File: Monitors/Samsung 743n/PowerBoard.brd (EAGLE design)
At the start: 160 x 128 mm, 60 parts, among them IC2 HV9961NG-G, T1 TRANS-1/1EFD25-10, X1 CON-MONPANEL, X2 CON-2MM-12P

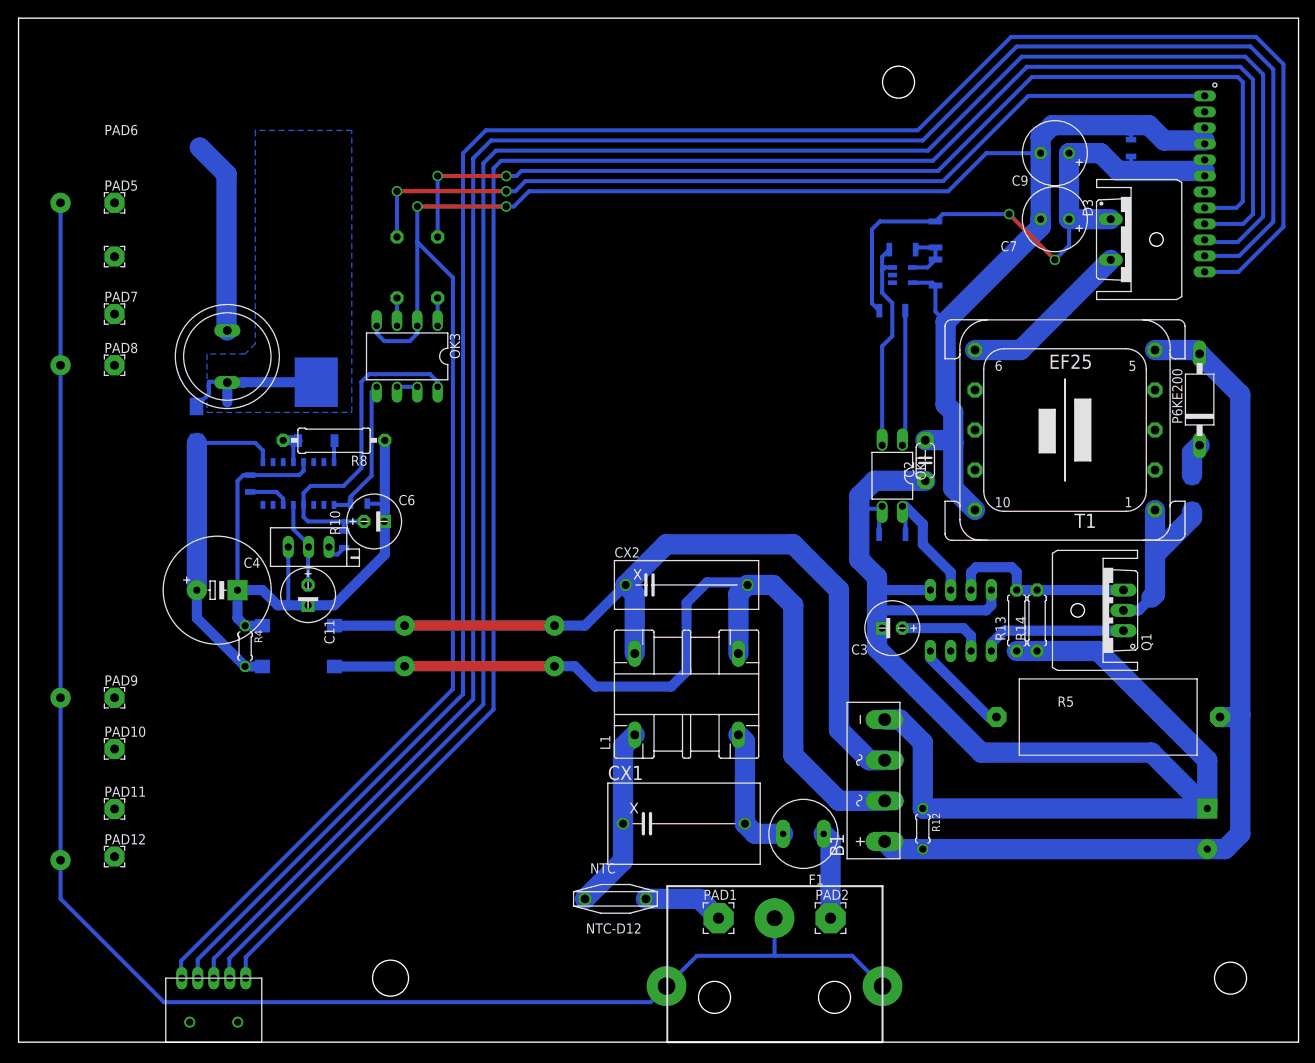
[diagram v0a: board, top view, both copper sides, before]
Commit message: Релиз
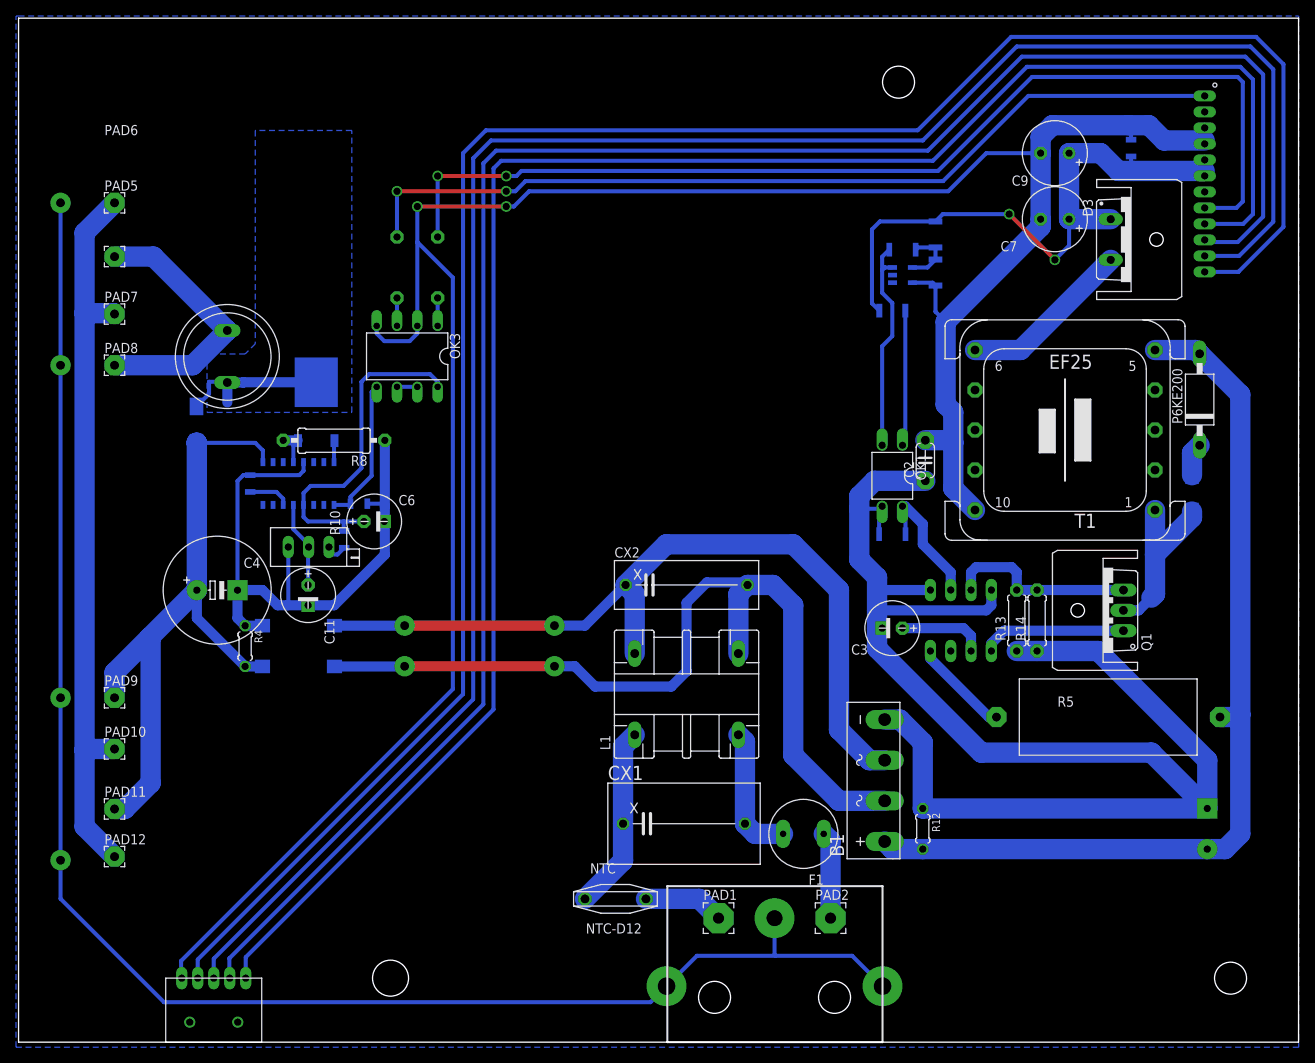
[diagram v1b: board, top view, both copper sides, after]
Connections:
- new net N$3: PAD10.1, PAD12.1, PAD5.1, PAD7.1
- net LED+: now also PAD11.1, PAD9.1
- net LED-: now also PAD6.1, PAD8.1
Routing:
- net N$3: track 0.00 -> 92.4 mm
- net LED+: track 42.7 -> 84.6 mm
- net LED-: track 24.3 -> 34.0 mm
- added copper zone on layer 16, net GROUND
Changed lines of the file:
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@@
 <wire x1="28.3225" y1="46.97" x2="22.29" y2="53.0025" width="1.27" layer="16"/>
 <wire x1="22.29" y1="53.0025" x2="22.29" y2="56.495" width="1.27" layer="16"/>
-<wire x1="22.29" y1="74.91" x2="22.245" y2="74.9325" width="0" layer="19" extent="16-16"/>
+<contactref element="PAD9" pad="1"/>
+<contactref element="PAD11" pad="1"/>
+<wire x1="12" y1="43.0475" x2="12" y2="46.205" width="2.54" layer="16"/>
+<wire x1="12" y1="46.205" x2="16.39375" y2="50.59875" width="2.54" layer="16"/>
+<wire x1="16.39375" y1="50.59875" x2="22.29" y2="56.495" width="2.54" layer="16"/>
+<wire x1="12" y1="29.1475" x2="13.2725" y2="29.1475" width="2.54" layer="16"/>
+<wire x1="13.2725" y1="29.1475" x2="16.51" y2="32.385" width="2.54" layer="16"/>
+<wire x1="16.51" y1="32.385" x2="16.51" y2="50.4825" width="2.54" layer="16"/>
+<wire x1="16.51" y1="50.4825" x2="16.39375" y2="50.59875" width="2.54" layer="16"/>
+<wire x1="22.245" y1="74.9325" x2="22.2675" y2="74.9325" width="2.54" layer="16"/>
+<wire x1="22.2675" y1="74.9325" x2="22.29" y2="74.91" width="2.54" layer="16"/>
 </signal>
 <signal name="LED-">
 <contactref element="L2" pad="P$2"/>
-<wire x1="22.65" y1="111.85" x2="26" y2="108.5" width="2.54" layer="16"/>
-<wire x1="26" y1="108.5" x2="26" y2="89.055" width="2.54" layer="16"/>
 <wire x1="26" y1="89.055" x2="26.1" y2="88.955" width="2.54" layer="16"/>
+<contactref element="PAD8" pad="1"/>
+<contactref element="PAD6" pad="1"/>
+<wire x1="26.1" y1="88.955" x2="16.8575" y2="98.1975" width="2.54" layer="16"/>
+<wire x1="16.8575" y1="98.1975" x2="12" y2="98.1975" width="2.54" layer="16"/>
+<wire x1="12" y1="84.615" x2="21.76" y2="84.615" width="2.54" layer="16"/>
+<wire x1="21.76" y1="84.615" x2="26.1" y2="88.955" width="2.54" layer="16"/>
 </signal>
 <signal name="N$7">
@@
 <wire x1="5.25" y1="17.9275" x2="18.1815" y2="4.996" width="0.508" layer="16"/>
 <wire x1="78.996" y1="4.996" x2="81" y2="7" width="0.508" layer="16"/>
+<polygon width="0.4064" layer="16" isolate="1.27" orphans="yes" rank="6">
+<vertex x="0" y="128.27"/>
+<vertex x="160.02" y="128.27"/>
+<vertex x="160.02" y="-0.635"/>
+<vertex x="-0.3175" y="-0.635"/>
+<vertex x="-0.3175" y="127.9525"/>
+<vertex x="-0.3175" y="128.27"/>
+</polygon>
 </signal>
 <signal name="K2">
@@
 <contactref element="X2" pad="7"/>
 </signal>
+<signal name="N$3">
+<contactref element="PAD7" pad="1"/>
+<contactref element="PAD5" pad="1"/>
+<contactref element="PAD10" pad="1"/>
+<contactref element="PAD12" pad="1"/>
+<wire x1="12" y1="104.915" x2="8.255" y2="101.17" width="2.54" layer="16"/>
+<wire x1="8.255" y1="26.9425" x2="12" y2="23.1975" width="2.54" layer="16"/>
+<wire x1="8.255" y1="101.17" x2="8.255" y2="91.1225" width="2.54" layer="16"/>
+<wire x1="8.255" y1="91.1225" x2="8.255" y2="36.5125" width="2.54" layer="16"/>
+<wire x1="8.255" y1="36.5125" x2="8.255" y2="26.9425" width="2.54" layer="16"/>
+<wire x1="12" y1="36.6475" x2="8.39" y2="36.6475" width="2.54" layer="16"/>
+<wire x1="8.39" y1="36.6475" x2="8.255" y2="36.5125" width="2.54" layer="16"/>
+<wire x1="12" y1="91.015" x2="11.8925" y2="91.1225" width="2.54" layer="16"/>
+<wire x1="11.8925" y1="91.1225" x2="8.255" y2="91.1225" width="2.54" layer="16"/>
+</signal>
 </signals>

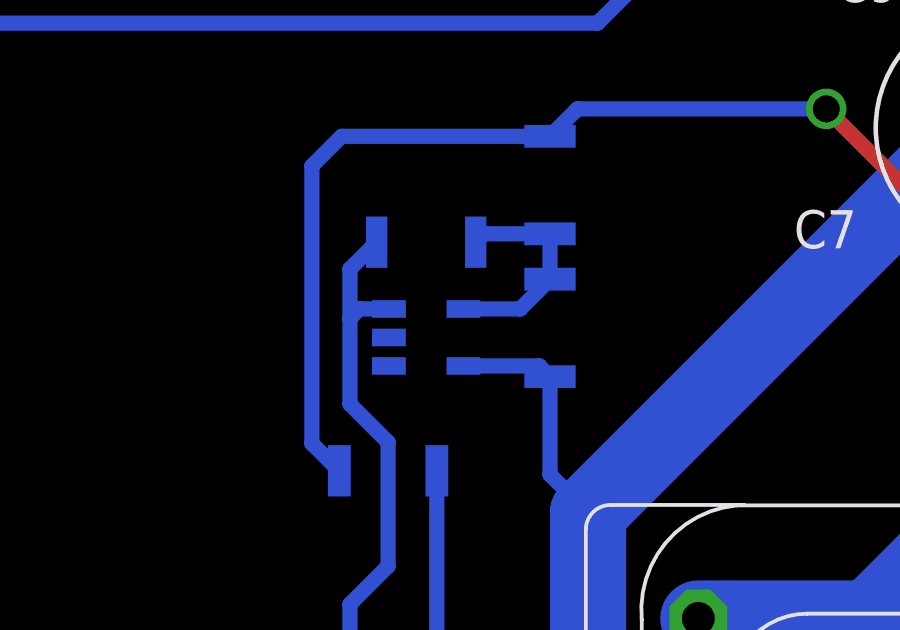
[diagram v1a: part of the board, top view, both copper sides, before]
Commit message: _)
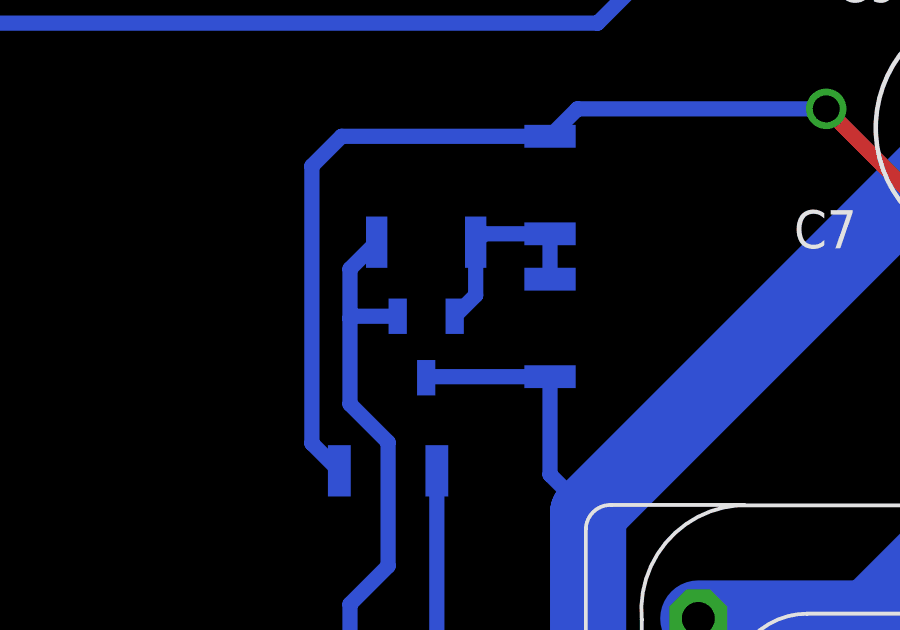
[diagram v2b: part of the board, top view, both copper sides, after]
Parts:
- U$3: value IC-TL431DBV -> IC-TL431CDBZR; device Flamberm:SOT95P280X145-5 -> Flamberm:SOT95P240X115-3
- moved U$3 0.32 mm to (110.5, 95.6), turned to 270 degrees
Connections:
- net GND: now also U$3.3; no longer U$3.5
- net N$23: now also U$3.2; no longer U$3.4
- net N$31: now also U$3.1; no longer U$3.3
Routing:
- net GND: track 302.6 -> 303.7 mm
- net N$23: track 7.40 -> 6.86 mm
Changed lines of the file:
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@@
 </layers>
 <board>
+<fusionsync huburn="a.cGVyc29uYWw6dWUyOGRlMGUz" projecturn="a.cGVyc29uYWw6dWUyOGRlMGUzIzIwMTgxMjA3MTY0MzUzMzMx" f3durn="urn:adsk.wipprod:dm.lineage:CbOk_p9-Sm28mP2tJHSDlw" pcbguid="25285c78-3eb6-47c6-8325-666efd53a6fb" lastpulledtime="" lastsyncedchangeguid="d28009d4-24da-5f07-1719-9be39d882890"/>
 <plain>
 <wire x1="0" y1="0" x2="160" y2="0" width="0" layer="20"/>
@@
 <attribute name="VALUE" x="132.6642" y="106.0958" size="1.27" layer="27" ratio="10" rot="R180"/>
 </element>
-<element name="U$3" library="Flamberm" library_urn="urn:adsk.eagle:library:2654185" package="SOT95P280X145-5" package3d_urn="urn:adsk.eagle:package:4135333/1" value="IC-TL431DBV" x="110.49" y="95.885" smashed="yes" rot="MR180">
-<attribute name="NAME" x="108.712" y="98.933" size="1.27" layer="26" ratio="10" rot="MR270"/>
-<attribute name="VALUE" x="113.538" y="98.933" size="1.27" layer="28" ratio="10" rot="MR270"/>
+<element name="U$3" library="Flamberm" library_urn="urn:adsk.eagle:library:2654185" package="SOT95P240X115-3" package3d_urn="urn:adsk.eagle:package:4135509/1" value="IC-TL431CDBZR" x="110.49" y="95.5675" smashed="yes" rot="MR270">
+<attribute name="NAME" x="113.538" y="97.3455" size="1.27" layer="26" ratio="10" rot="MR0"/>
+<attribute name="VALUE" x="113.538" y="92.5195" size="1.27" layer="28" ratio="10" rot="MR0"/>
 </element>
 <element name="R7" library="Flamberm" library_urn="urn:adsk.eagle:library:2654185" package="RESC3216X60" package3d_urn="urn:adsk.eagle:package:4015759/1" value="220R" x="109.22" y="91.44" smashed="yes" rot="MR0">
@@
 <wire x1="49.8475" y1="88.5825" x2="49.8475" y2="89.535" width="0.508" layer="16"/>
 <contactref element="C2" pad="2"/>
-<contactref element="U$3" pad="5"/>
+<contactref element="U$3" pad="3"/>
 <contactref element="R18" pad="1"/>
 <contactref element="C7" pad="-"/>
@@
 <wire x1="114.6175" y1="94.5775" x2="114.6175" y2="91.313" width="0.508" layer="16"/>
 <wire x1="114.6175" y1="91.313" x2="115.8875" y2="90.043" width="0.508" layer="16"/>
-<wire x1="111.7321" y1="94.935" x2="114.26" y2="94.935" width="0.508" layer="16"/>
-<wire x1="114.26" y1="94.935" x2="114.6175" y2="94.5775" width="0.508" layer="16"/>
 <wire x1="127.762" y1="111.125" x2="120.9675" y2="111.125" width="0.508" layer="16"/>
 <wire x1="120.9675" y1="111.125" x2="116.205" y2="106.3625" width="0.508" layer="16"/>
@@
 <wire x1="63.8175" y1="106.3625" x2="61.9125" y2="104.4575" width="0.508" layer="16"/>
 <wire x1="60.96" y1="104.4575" x2="49.8475" y2="104.4575" width="0.508" layer="1"/>
+<wire x1="114.6175" y1="94.5775" x2="110.5245" y2="94.5775" width="0.508" layer="16"/>
+<wire x1="110.5245" y1="94.5775" x2="110.49" y2="94.543" width="0.508" layer="16"/>
 </signal>
 <signal name="+5V">
@@
 <signal name="N$31">
 <contactref element="OK1" pad="2"/>
-<contactref element="U$3" pad="3"/>
+<contactref element="U$3" pad="1"/>
 <contactref element="C8" pad="1"/>
-<wire x1="107.95" y1="96.52" x2="108.2675" y2="96.8375" width="0.508" layer="16"/>
-<wire x1="108.2675" y1="96.8375" x2="108.27" y2="96.835" width="0.508" layer="16"/>
-<wire x1="108.27" y1="96.835" x2="109.2479" y2="96.835" width="0.508" layer="16"/>
 <wire x1="108.84" y1="99.06" x2="107.95" y2="98.17" width="0.508" layer="16"/>
-<wire x1="107.95" y1="98.17" x2="107.95" y2="96.52" width="0.508" layer="16"/>
 <wire x1="107.95" y1="93.6625" x2="109.22" y2="92.3925" width="0.508" layer="16"/>
 <wire x1="109.22" y1="92.3925" x2="109.22" y2="88.265" width="0.508" layer="16"/>
 <wire x1="109.22" y1="88.265" x2="107.95" y2="86.995" width="0.508" layer="16"/>
 <wire x1="107.95" y1="86.995" x2="107.95" y2="74.6125" width="0.508" layer="16"/>
+<wire x1="107.95" y1="98.17" x2="107.95" y2="96.52" width="0.508" layer="16"/>
 <wire x1="107.95" y1="96.52" x2="107.95" y2="93.6625" width="0.508" layer="16"/>
+<wire x1="107.95" y1="96.52" x2="108.022" y2="96.592" width="0.508" layer="16"/>
+<wire x1="108.022" y1="96.592" x2="109.54" y2="96.592" width="0.508" layer="16"/>
 </signal>
 <signal name="N$22">
@@
 </signal>
 <signal name="N$23">
-<contactref element="U$3" pad="4"/>
+<contactref element="U$3" pad="2"/>
 <contactref element="R11" pad="1"/>
 <contactref element="C8" pad="2"/>
@@
 <wire x1="112.42" y1="99.34" x2="114.6175" y2="99.34" width="0.508" layer="16"/>
 <wire x1="114.6175" y1="97.8275" x2="114.6175" y2="99.34" width="0.508" layer="16"/>
-<wire x1="111.7321" y1="96.835" x2="113.625" y2="96.835" width="0.508" layer="16"/>
-<wire x1="113.625" y1="96.835" x2="114.6175" y2="97.8275" width="0.508" layer="16"/>
+<wire x1="111.44" y1="96.592" x2="112.14" y2="97.292" width="0.508" layer="16"/>
+<wire x1="112.14" y1="97.292" x2="112.14" y2="99.06" width="0.508" layer="16"/>
 </signal>
 <signal name="N$30">
@@
 </note>
 <note version="8.3" severity="warning">
+Since Version 8.3, EAGLE supports Fusion synchronisation.
+This feature will not be available in this version and saving
+the document will break the link to the Fusion PCB feature.
+</note>
+<note version="8.3" severity="warning">
